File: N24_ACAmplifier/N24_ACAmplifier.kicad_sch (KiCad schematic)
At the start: 24 parts

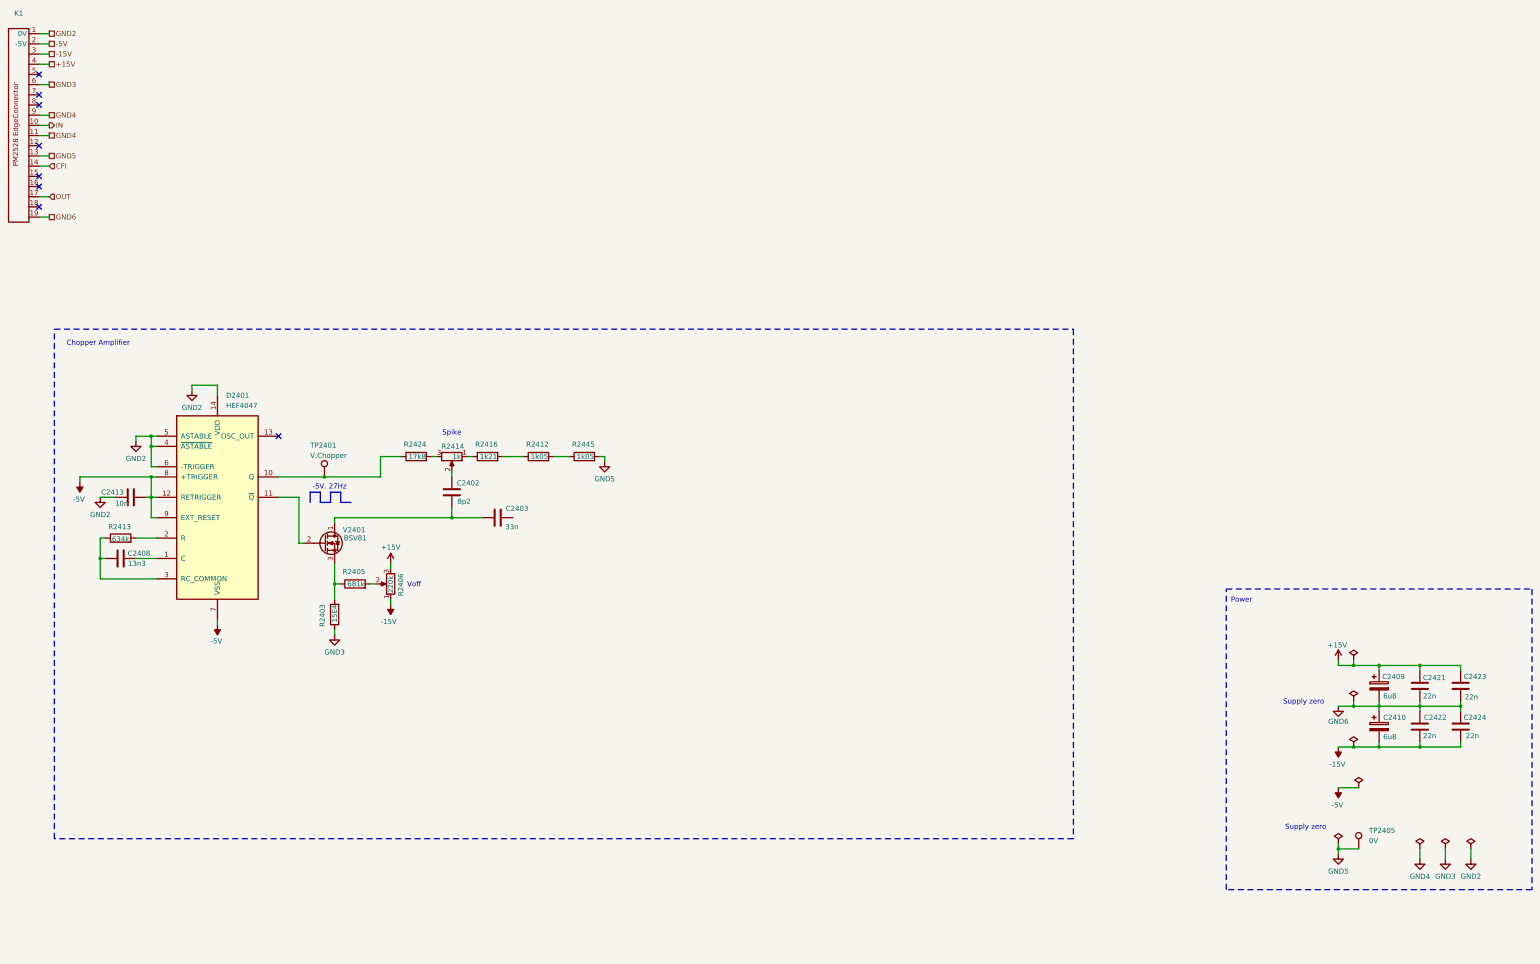
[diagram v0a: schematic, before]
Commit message: Small updates, N25 also
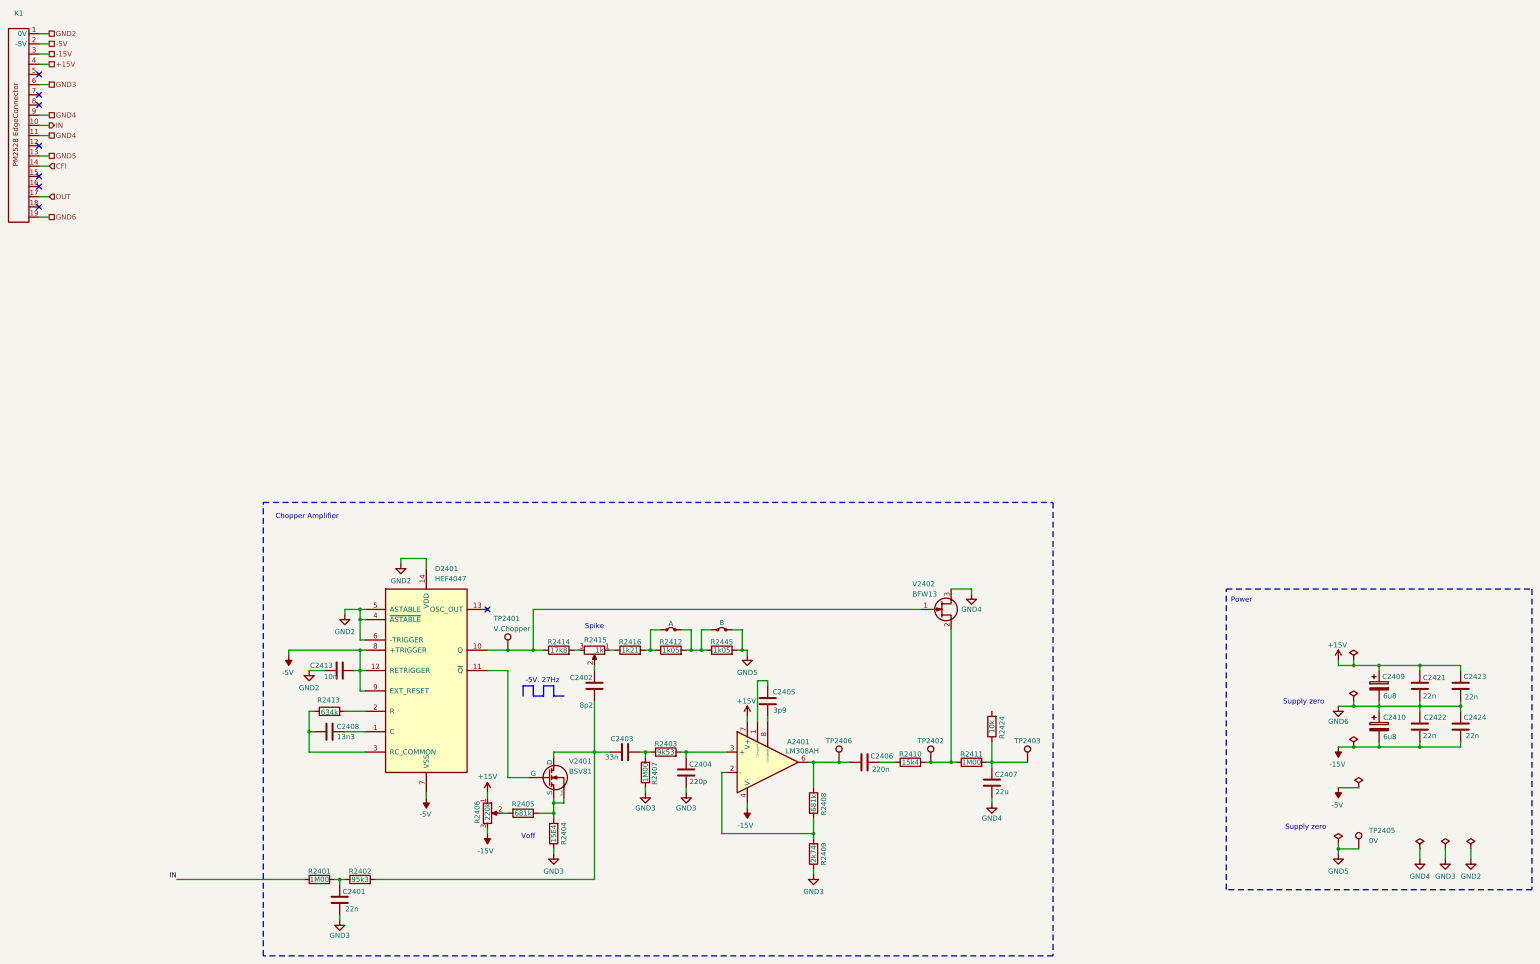
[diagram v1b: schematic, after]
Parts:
- removed V2401: BSV81, Package_TO_SOT_THT:TO-92_Inline, symbol Transistor_FET:BS108
- added A2401: LM308AH, Package_DIP:DIP-8_W7.62mm, symbol PM2528:OPAMP_COMPEN
- added C2401: 22n, symbol Device:C
- added C2404: 220p, symbol Device:C
- added C2405: 3p9, symbol Device:C
- added C2406: 220n, symbol Device:C
- added C2407: 22u, symbol Device:C
- added JP1: A, TestPoint:TestPoint_Bridge_Pitch2.54mm_Drill1.0mm, symbol Jumper:Jumper_2_Small_Bridged
- added JP2: B, TestPoint:TestPoint_Bridge_Pitch2.54mm_Drill1.0mm, symbol Jumper:Jumper_2_Small_Bridged
- added R2401, R2407, R2411: 1M00, symbol Device:R
- added R2402: 95k3, symbol Device:R
- added R2403: 9k53, symbol Device:R
- added R2408: 681k, symbol Device:R
- added R2409: 2k74, symbol Device:R
- added R2410: 15k4, symbol Device:R
- added R2424: 10k, symbol Device:R
- added TP2402, TP2403: ~, TestPoint:TestPoint_Loop_D2.50mm_Drill1.0mm, symbol Connector:TestPoint
- added TP2406: AC_RMS?, TestPoint:TestPoint_Loop_D2.50mm_Drill1.0mm, symbol Connector:TestPoint
- added V2401: BSV81, Package_TO_SOT_THT:TO-72-4, symbol Simulation_SPICE:NMOS_Substrate
- added V2402: BFW13, Package_TO_SOT_THT:TO-72-4, symbol Transistor_FET:BF245C
- D2401: footprint (none) -> Package_DIP:DIP-14_W7.62mm
- TP2401, TP2405: footprint (none) -> TestPoint:TestPoint_Loop_D2.50mm_Drill1.0mm
- renumbered R2403 to R2404, R2424 to R2414, R2414 to R2415
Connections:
- net +15V: now also R2406.1, A2401.7 (V+); no longer R2406.3
- net -15V: now also R2406.3, A2401.4 (V-); no longer R2406.1
- net GND3: now also C2401.2, C2404.2, R2407.1, R2409.1
- net GND4: now also C2407.2, V2402.3 (D)
- net GND5: now also JP2.2 (B)
- net IN: now also R2401.1
- net at R2412.1, R2416.2: now also JP1.1 (A)
- net at R2412.2, R2445.1: now also JP1.2 (B), JP2.1 (A)
- net at R2404.2, R2405.1: now also V2401.3 (S), V2401.4 (Bulk)
- net at D2401.10 (Q), R2414.1, TP2401.1: now also V2402.1 (G)
- net at C2402.2, C2403.1: now also R2402.2, V2401.1 (D)
- net at C2403.2: now also R2403.1, R2407.2
- net at D2401.11 (~{Q}): now also V2401.2 (G)
- new net: C2407.1, R2411.2, R2424.1, TP2403.1
- new net: A2401.6, C2406.1, R2408.2, TP2406.1
- new net: C2406.2, R2410.1
- new net: R2410.2, R2411.1, TP2402.1, V2402.2 (S)
- new net: C2401.1, R2401.2, R2402.1
- new net: A2401.2 (-), R2408.1, R2409.2
- new net: A2401.3 (+), C2404.1, R2403.2
- new net: A2401.1 (CompenA), C2405.1
- new net: A2401.8 (CompenB), C2405.2
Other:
- moved on the sheet: C2402, C2403, C2408, C2413, D2401, R2404, R2405, R2406, R2412, R2413, R2414, R2415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
